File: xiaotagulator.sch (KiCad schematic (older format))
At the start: 15 parts, among them J1 JTAG, J2 UART, J3 Conn_01x05, U1 SeeeduinoXIAO

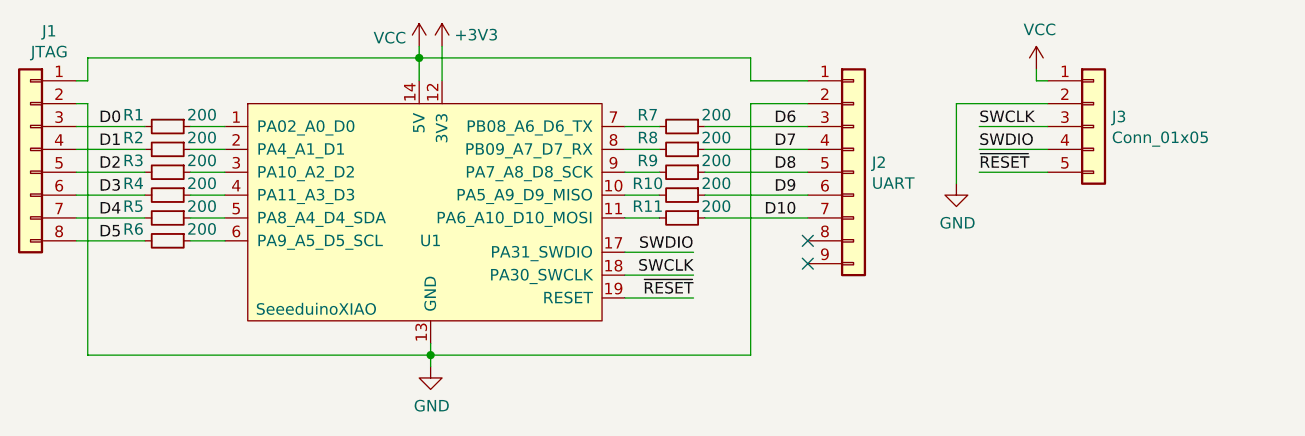
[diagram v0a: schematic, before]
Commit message: Feedback
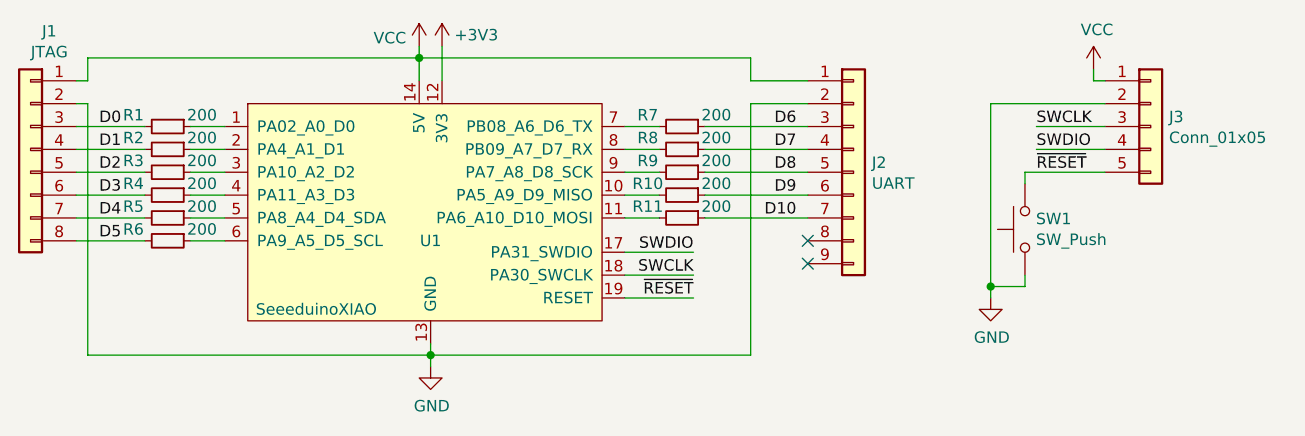
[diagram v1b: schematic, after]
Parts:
- added SW1: SW_Push, Button_Switch_SMD:SW_SPST_B3U-1000P, symbol Switch:SW_Push
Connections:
- net GND: now also SW1.1
- net ~RESET: now also SW1.2
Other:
- moved on the sheet: J3
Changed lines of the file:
@@
 L Connector_Generic:Conn_01x05 J3
 U 1 1 6143CA3E
-P 5600 1250
-F 0 "J3" H 5680 1292 50  0000 L CNN
-F 1 "Conn_01x05" H 5680 1201 50  0000 L CNN
-F 2 "Connector_PinHeader_2.54mm:PinHeader_1x05_P2.54mm_Vertical" H 5600 1250 50  0001 C CNN
-F 3 "~" H 5600 1250 50  0001 C CNN
-	1    5600 1250
+P 5850 1250
+F 0 "J3" H 5930 1292 50  0000 L CNN
+F 1 "Conn_01x05" H 5930 1201 50  0000 L CNN
+F 2 "Connector_PinHeader_2.54mm:PinHeader_1x05_P2.54mm_Vertical" H 5850 1250 50  0001 C CNN
+F 3 "~" H 5850 1250 50  0001 C CNN
+	1    5850 1250
 	1    0    0    -1
 $EndComp
@@
 L power:VCC #PWR0101
 U 1 1 6144003B
-P 5350 1000
-F 0 "#PWR0101" H 5350 850 50  0001 C CNN
-F 1 "VCC" H 5365 1173 50  0000 C CNN
-F 2 "" H 5350 1000 50  0001 C CNN
-F 3 "" H 5350 1000 50  0001 C CNN
-	1    5350 1000
+P 5600 1000
+F 0 "#PWR0101" H 5600 850 50  0001 C CNN
+F 1 "VCC" H 5615 1173 50  0000 C CNN
+F 2 "" H 5600 1000 50  0001 C CNN
+F 3 "" H 5600 1000 50  0001 C CNN
+	1    5600 1000
 	1    0    0    -1
 $EndComp
 Wire Wire Line
-	5350 1000 5350 1050
+	5600 1000 5600 1050
 Wire Wire Line
-	5350 1050 5400 1050
-Text Label 5100 1250 0    50   ~ 0
+	5600 1050 5650 1050
+Text Label 5350 1250 0    50   ~ 0
 SWCLK
 Wire Wire Line
-	5100 1250 5400 1250
-Text Label 5100 1350 0    50   ~ 0
+	5350 1250 5650 1250
+Text Label 5350 1350 0    50   ~ 0
 SWDIO
 Wire Wire Line
-	5100 1350 5400 1350
-Text Label 5100 1450 0    50   ~ 0
+	5350 1350 5650 1350
+Text Label 5350 1450 0    50   ~ 0
 ~RESET
-Wire Wire Line
-	5100 1450 5400 1450
 $Comp
 L power:GND #PWR0102
 U 1 1 61443FE0
-P 5000 1500
-F 0 "#PWR0102" H 5000 1250 50  0001 C CNN
-F 1 "GND" H 5005 1327 50  0000 C CNN
-F 2 "" H 5000 1500 50  0001 C CNN
-F 3 "" H 5000 1500 50  0001 C CNN
-	1    5000 1500
+P 5150 2000
+F 0 "#PWR0102" H 5150 1750 50  0001 C CNN
+F 1 "GND" H 5155 1827 50  0000 C CNN
+F 2 "" H 5150 2000 50  0001 C CNN
+F 3 "" H 5150 2000 50  0001 C CNN
+	1    5150 2000
 	1    0    0    -1
 $EndComp
 Wire Wire Line
-	5000 1500 5000 1150
+	5150 2000 5150 1950
 Wire Wire Line
-	5000 1150 5400 1150
+	5150 1150 5650 1150
 Text Label 1250 1250 0    50   ~ 0
 D0
@@
 Text Label 4300 1650 2    50   ~ 0
 D10
+$Comp
+L Switch:SW_Push SW1
+U 1 1 613FE241
+P 5300 1700
+F 0 "SW1" V 5346 1652 50  0000 R CNN
+F 1 "SW_Push" V 5255 1652 50  0000 R CNN
+F 2 "Button_Switch_SMD:SW_SPST_B3U-1000P" H 5300 1900 50  0001 C CNN
+F 3 "~" H 5300 1900 50  0001 C CNN
+	1    5300 1700
+	0    -1   -1   0
+$EndComp
+Wire Wire Line
+	5300 1500 5300 1450
+Wire Wire Line
+	5300 1450 5650 1450
+Wire Wire Line
+	5300 1900 5300 1950
+Wire Wire Line
+	5300 1950 5150 1950
+Connection ~ 5150 1950
+Wire Wire Line
+	5150 1950 5150 1150
 $EndSCHEMATC

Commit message: Last adjustments before prototype order
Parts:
- J1: LCSC (none) -> C225494
- J2: LCSC (none) -> C225495
- R1, R10, R11, R2, R3, R4, R5, R6, R7, R8, R9: LCSC (none) -> C8218
- SW1: LCSC (none) -> C498294
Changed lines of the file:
@@
 F 2 "Resistor_SMD:R_0603_1608Metric" H 3800 1250 50  0001 C CNN
 F 3 "~" H 3800 1250 50  0001 C CNN
+F 4 "C8218" H 3800 1250 50  0001 C CNN "LCSC"
 	1    3800 1250
 	0    1    1    0
@@
 F 2 "Resistor_SMD:R_0603_1608Metric" H 3800 1350 50  0001 C CNN
 F 3 "~" H 3800 1350 50  0001 C CNN
+F 4 "C8218" H 3800 1350 50  0001 C CNN "LCSC"
 	1    3800 1350
 	0    1    1    0
@@
 F 2 "Resistor_SMD:R_0603_1608Metric" H 3800 1450 50  0001 C CNN
 F 3 "~" H 3800 1450 50  0001 C CNN
+F 4 "C8218" H 3800 1450 50  0001 C CNN "LCSC"
 	1    3800 1450
 	0    1    1    0
@@
 F 2 "Resistor_SMD:R_0603_1608Metric" H 3800 1550 50  0001 C CNN
 F 3 "~" H 3800 1550 50  0001 C CNN
+F 4 "C8218" H 3800 1550 50  0001 C CNN "LCSC"
 	1    3800 1550
 	0    1    1    0
@@
 F 2 "Resistor_SMD:R_0603_1608Metric" H 3800 1650 50  0001 C CNN
 F 3 "~" H 3800 1650 50  0001 C CNN
+F 4 "C8218" H 3800 1650 50  0001 C CNN "LCSC"
 	1    3800 1650
 	0    1    1    0
@@
 F 2 "Connector_PinHeader_2.54mm:PinHeader_1x09_P2.54mm_Horizontal" H 4550 1450 50  0001 C CNN
 F 3 "~" H 4550 1450 50  0001 C CNN
+F 4 "C225495" H 4550 1450 50  0001 C CNN "LCSC"
 	1    4550 1450
 	1    0    0    -1
@@
 F 2 "Resistor_SMD:R_0603_1608Metric" H 1550 1250 50  0001 C CNN
 F 3 "~" H 1550 1250 50  0001 C CNN
+F 4 "C8218" H 1550 1250 50  0001 C CNN "LCSC"
 	1    1550 1250
 	0    1    1    0
@@
 F 2 "Resistor_SMD:R_0603_1608Metric" H 1550 1350 50  0001 C CNN
 F 3 "~" H 1550 1350 50  0001 C CNN
+F 4 "C8218" H 1550 1350 50  0001 C CNN "LCSC"
 	1    1550 1350
 	0    1    1    0
@@
 F 2 "Resistor_SMD:R_0603_1608Metric" H 1550 1450 50  0001 C CNN
 F 3 "~" H 1550 1450 50  0001 C CNN
+F 4 "C8218" H 1550 1450 50  0001 C CNN "LCSC"
 	1    1550 1450
 	0    1    1    0
@@
 F 2 "Resistor_SMD:R_0603_1608Metric" H 1550 1550 50  0001 C CNN
 F 3 "~" H 1550 1550 50  0001 C CNN
+F 4 "C8218" H 1550 1550 50  0001 C CNN "LCSC"
 	1    1550 1550
 	0    1    1    0
@@
 F 2 "Resistor_SMD:R_0603_1608Metric" H 1550 1650 50  0001 C CNN
 F 3 "~" H 1550 1650 50  0001 C CNN
+F 4 "C8218" H 1550 1650 50  0001 C CNN "LCSC"
 	1    1550 1650
 	0    1    1    0
@@
 F 2 "Resistor_SMD:R_0603_1608Metric" H 1550 1750 50  0001 C CNN
 F 3 "~" H 1550 1750 50  0001 C CNN
+F 4 "C8218" H 1550 1750 50  0001 C CNN "LCSC"
 	1    1550 1750
 	0    1    1    0
@@
 F 2 "Connector_PinHeader_2.54mm:PinHeader_1x08_P2.54mm_Horizontal" H 950 1350 50  0001 C CNN
 F 3 "~" H 950 1350 50  0001 C CNN
+F 4 "C225494" H 950 1350 50  0001 C CNN "LCSC"
 	1    950  1350
 	-1   0    0    -1
@@
 F 2 "Button_Switch_SMD:SW_SPST_B3U-1000P" H 5300 1900 50  0001 C CNN
 F 3 "~" H 5300 1900 50  0001 C CNN
+F 4 "C498294" H 5300 1700 50  0001 C CNN "LCSC"
 	1    5300 1700
 	0    -1   -1   0
